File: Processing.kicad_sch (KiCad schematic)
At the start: 48 parts

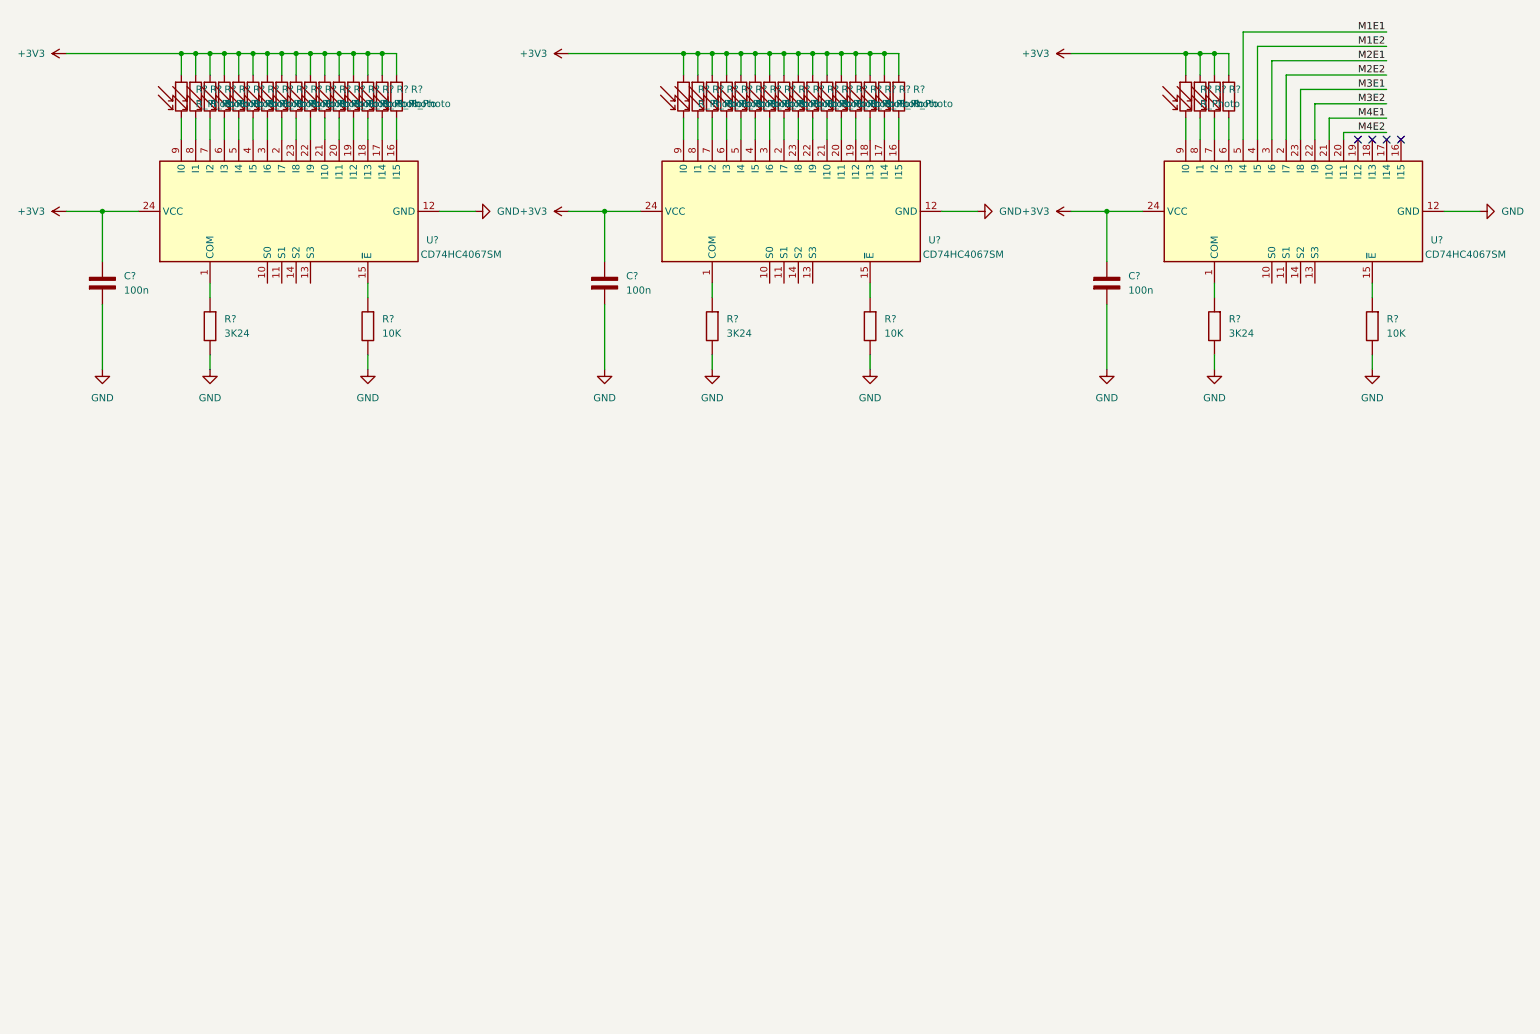
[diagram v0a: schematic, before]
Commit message: stm32
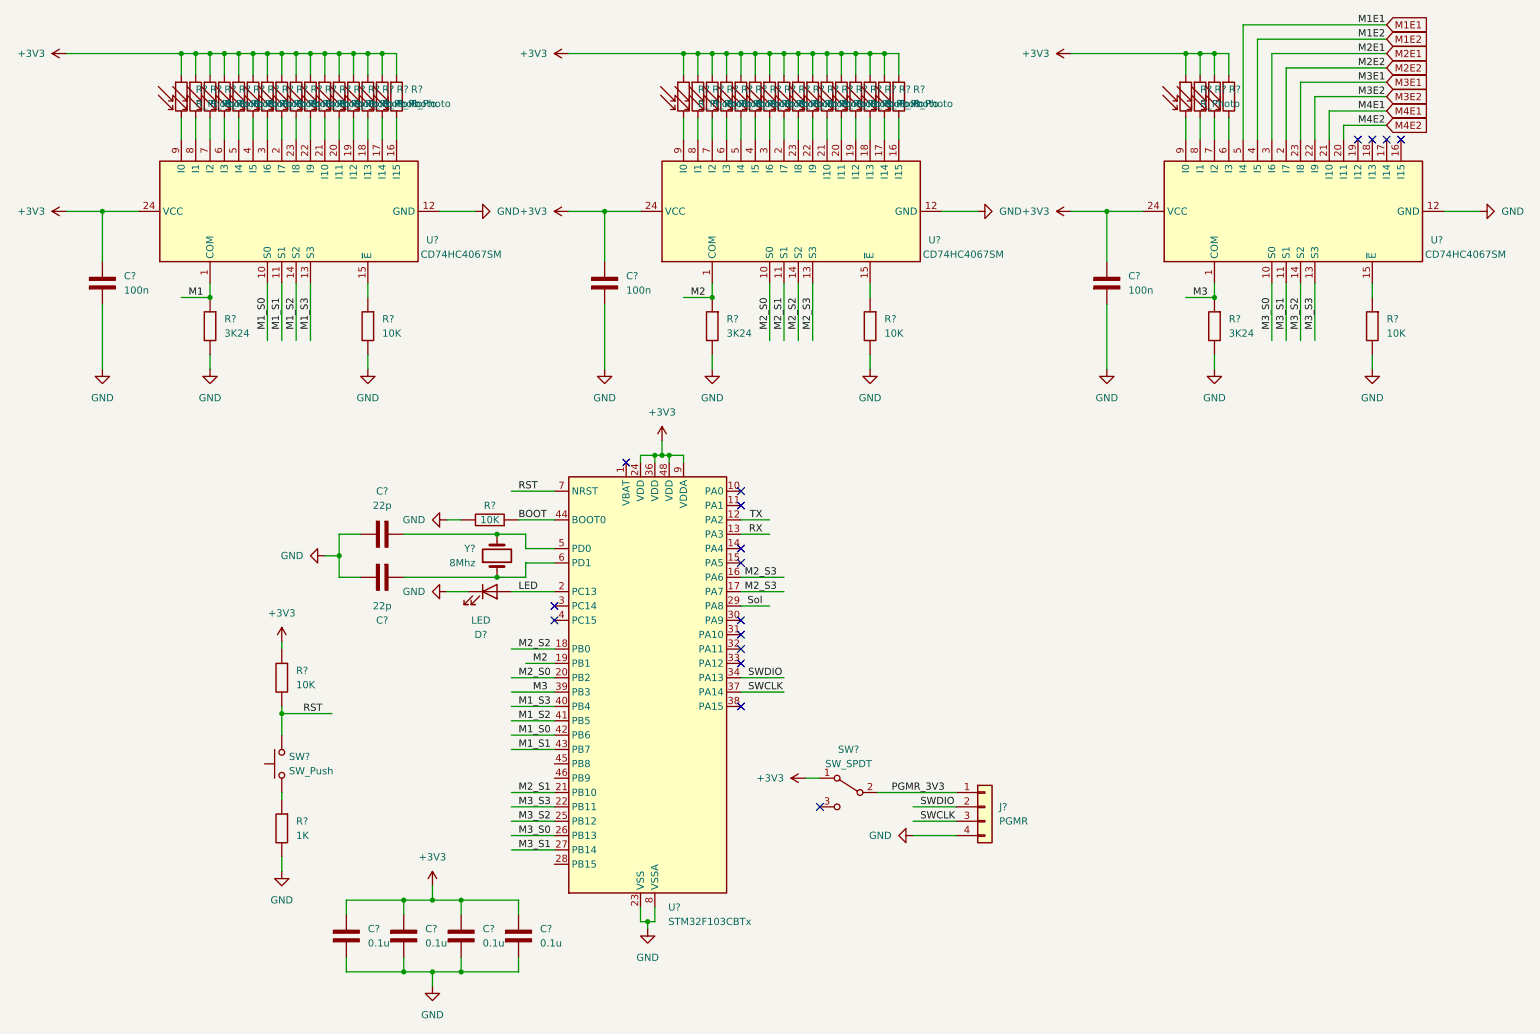
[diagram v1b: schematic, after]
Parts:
- added C? (x4): 0.1u, symbol vincent:C
- added C? (x2): 22p, symbol vincent:C
- added D?: LED, symbol Device:LED
- added J?: PGMR, symbol Connector_Generic:Conn_01x04
- added R? (x2): 10K, symbol vincent:R
- added R?: 1K, symbol vincent:R
- added SW?: SW_Push, symbol Switch:SW_Push
- added SW?: SW_SPDT, symbol Switch:SW_SPDT
- added U?: STM32F103CBTx, Package_QFP:LQFP-48_7x7mm_P0.5mm, symbol vincent:STM32F103CBTx
- added Y?: 8Mhz, symbol vincent:Crystal
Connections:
- net +3V3: now also C?.2, C?.2, C?.2, C?.2, R?.2, SW?.1 (A), U?.24 (VDD), U?.36 (VDD), U?.48 (VDD), U?.9 (VDDA)
- net GND: now also C?.1, C?.1, C?.1, C?.1, C?.1, C?.1, D?.1 (K), J?.4 (Pin_4), R?.1, R?.1, U?.23 (VSS), U?.35 (VSS), U?.47 (VSS), U?.8 (VSSA)
- net M1: now reaches R?.2, U?.1 (COM)
- net M3: now reaches R?.2, U?.1 (COM)
- net M3: now also U?.39 (PB3)
- net M3_S0: now reaches U?.10 (S0)
- net M3_S0: now also U?.26 (PB13)
- net M3_S1: now reaches U?.11 (S1)
- net M3_S1: now also U?.27 (PB14)
- net M3_S3: now reaches U?.13 (S3)
- net M3_S3: now also U?.22 (PB11)
- net M3_S2: now reaches U?.14 (S2)
- net M3_S2: now also U?.25 (PB12)
- net M2: now reaches R?.2, U?.1 (COM)
- net M2: now also U?.19 (PB1)
- net M2_S0: now reaches U?.10 (S0)
- net M2_S0: now also U?.20 (PB2)
- net M2_S1: now reaches U?.11 (S1)
- net M2_S1: now also U?.21 (PB10)
- net M2_S3: now reaches U?.13 (S3)
- net M2_S3: now also U?.16 (PA6), U?.17 (PA7)
- net M2_S2: now reaches U?.14 (S2)
- net M2_S2: now also U?.18 (PB0)
- net M1_S0: now reaches U?.10 (S0)
- net M1_S0: now also U?.42 (PB6)
- net M1_S1: now reaches U?.11 (S1)
- net M1_S1: now also U?.43 (PB7)
- net M1_S3: now reaches U?.13 (S3)
- net M1_S3: now also U?.40 (PB4)
- net M1_S2: now reaches U?.14 (S2)
- net M1_S2: now also U?.41 (PB5)
- new net: C?.2, U?.5 (PD0), Y?.2
- new net: C?.2, U?.6 (PD1), Y?.1
- new net: R?.2, SW?.1
- new net BOOT: R?.2, U?.44 (BOOT0)
- new net LED: D?.2 (A), U?.2 (PC13)
- new net PGMR_3V3: J?.1 (Pin_1), SW?.2 (B)
- new net RST: R?.1, SW?.2, U?.7 (NRST)
- new net RX: U?.13 (PA3)
- new net SWCLK: J?.3 (Pin_3), U?.37 (PA14)
- new net SWDIO: J?.2 (Pin_2), U?.34 (PA13)
- new net Sol: U?.29 (PA8)
- new net TX: U?.12 (PA2)
- no-connect marks 4 -> 17
